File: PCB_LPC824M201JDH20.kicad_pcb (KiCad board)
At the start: 2 copper layers, 15.2 x 25.4 mm, 9 parts, among them J1 Conn_01x10, J2 Conn_01x10, U1 LPC824M201JDH20

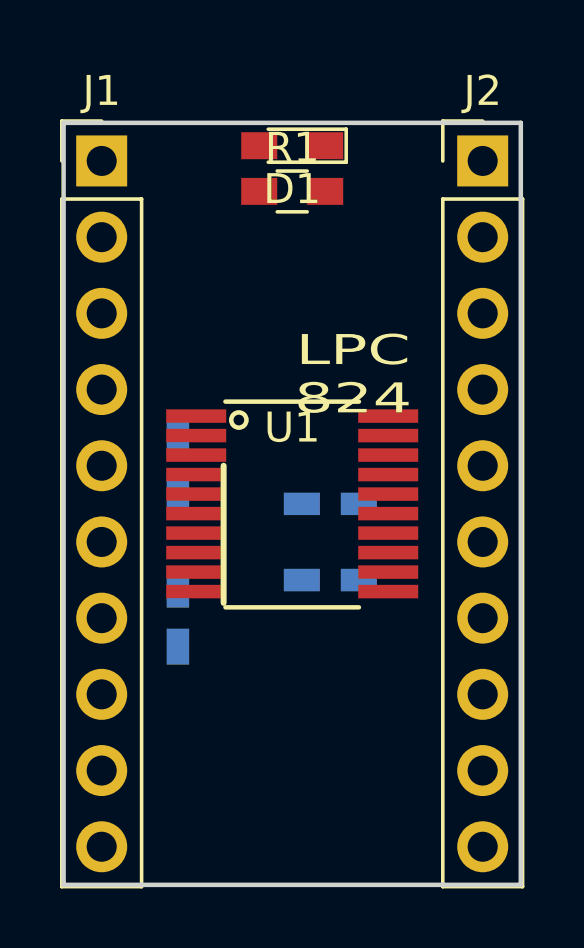
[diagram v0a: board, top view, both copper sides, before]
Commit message: no comment
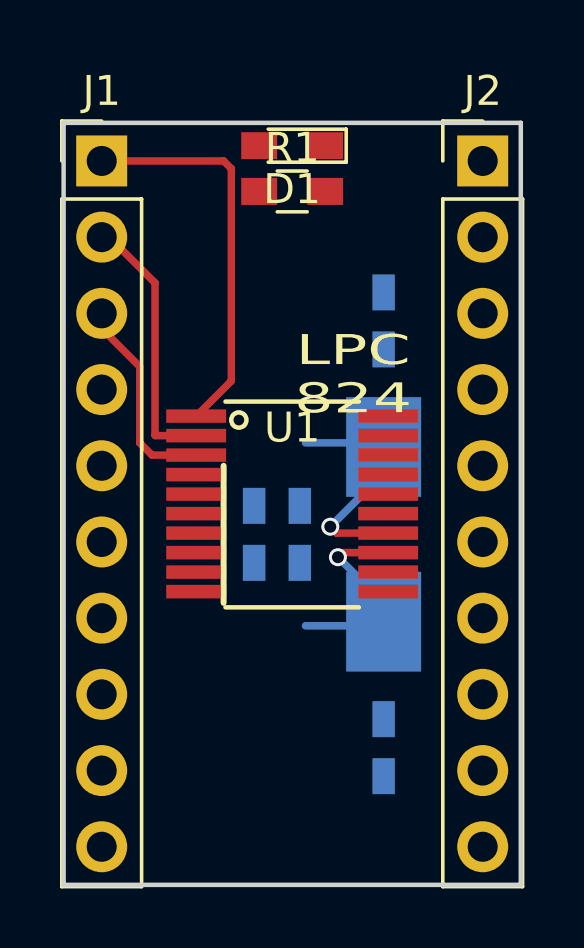
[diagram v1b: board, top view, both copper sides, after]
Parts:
- added 12MHz1: Crystal, Crystals:Crystal_SMD_0603-2pin_6.0x3.5mm_HandSoldering, B.Cu at (151.6, 111.5)
- moved C3 6.35 mm to (151.6, 104.4), turned to 270 degrees
- moved C4 5.86 mm to (151.6, 118.6), turned to 90 degrees
- moved C2 4.93 mm to (148.8, 111.5)
- moved C1 3.42 mm to (147.3, 111.5)
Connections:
- net Net-(J2-Pad3) renamed VREFP
- net Net-(J2-Pad4) renamed VREFN
- net Net-(J2-Pad5) renamed VSS
- net Net-(J2-Pad6) renamed VDD
- net RESET renamed PIO0_5
- J2 pad 1: Net-(J2-Pad1) -> PIO0_14
- J2 pad 10: Net-(J2-Pad10) -> PIO0_15
- J2 pad 2: Net-(J2-Pad2) -> PIO0_0
- J2 pad 7: Net-(J2-Pad7) -> XTALIN
- J2 pad 8: Net-(J2-Pad8) -> XTALOUT
- J2 pad 9: Net-(J2-Pad9) -> PIO0_1
- U1 pad 10: Net-(U1-Pad10) -> PIO0_10
- U1 pad 11: RFM_RST -> PIO0_15
- U1 pad 12: SCK -> PIO0_1
- U1 pad 19: RXD -> PIO0_0
- U1 pad 20: RFM_CS -> PIO0_14
- U1 pad 6: TXD -> PIO0_4
- U1 pad 7: SWCLK -> PIO0_3
- U1 pad 8: SWDIO -> PIO0_2
- U1 pad 9: FLASH_CS -> PIO0_11
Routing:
- net PIO0_23: track 0.00 -> 13.2 mm
- net PIO0_17: track 0.00 -> 8.87 mm
- net XTALIN: track 0.00 -> 8.08 mm, vias 0 -> 1
- net XTALOUT: track 0.00 -> 7.18 mm, vias 0 -> 1
- net PIO0_13: track 0.00 -> 6.89 mm

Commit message: no comment
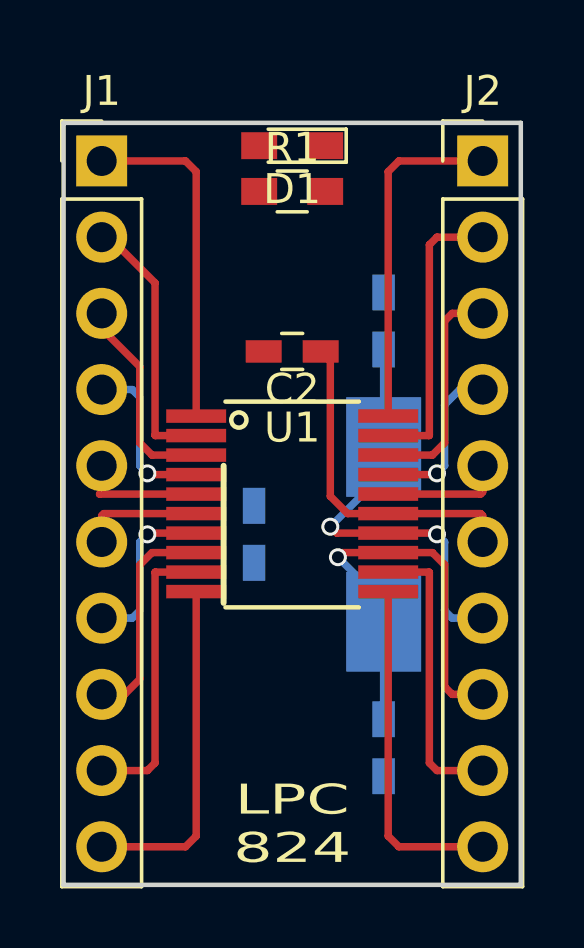
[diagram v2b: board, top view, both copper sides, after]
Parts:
- C2: moved to F.Cu
- moved C2 6.10 mm to (148.6, 105.4), turned to 180 degrees
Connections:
- J1 pad 5: PIO0_6 -> PIO0_5
- J2 pad 5: VSS -> GND
- J2 pad 6: VDD -> 3.3V
- U1 pad 17: GND -> VREFN
- U1 pad 18: 3.3V -> VREFP
- U1 pad 4: ISPE -> PIO0_12
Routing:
- net PIO0_14: track 0.00 -> 11.4 mm
- net PIO0_15: track 0.00 -> 11.4 mm
- net PIO0_10: track 0.00 -> 11.4 mm
- net 3.3V: track 0.00 -> 11.2 mm
- net PIO0_0: track 0.00 -> 9.61 mm
- net PIO0_1: track 0.00 -> 9.61 mm
- net PIO0_11: track 0.00 -> 9.61 mm
- net XTALOUT: track 7.18 -> 15.5 mm
- net VREFP: track 0.00 -> 7.49 mm
- net PIO0_2: track 0.00 -> 7.34 mm
- net XTALIN: track 8.08 -> 14.5 mm, vias 1 -> 2
- net PIO0_3: track 0.00 -> 5.66 mm, vias 0 -> 1
- net PIO0_12: track 0.00 -> 5.66 mm, vias 0 -> 1
- net VREFN: track 0.00 -> 5.51 mm, vias 0 -> 1
- net PIO0_5: track 0.00 -> 4.20 mm
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- added copper zone on B.Cu, net GND

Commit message: no comment
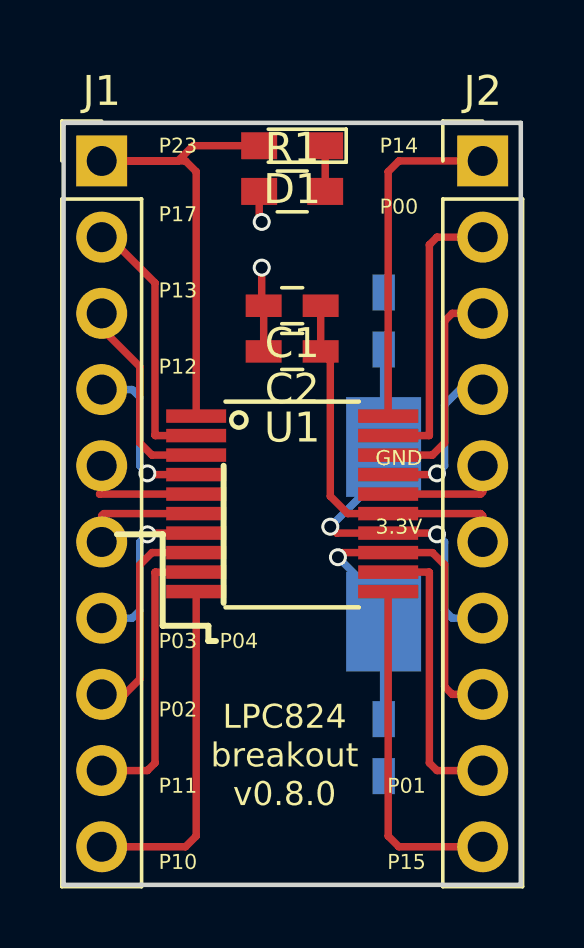
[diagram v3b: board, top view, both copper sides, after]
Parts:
- C1: moved to F.Cu
- moved C1 7.73 mm to (148.6, 103.9), turned to 180 degrees
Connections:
- J1 pad 1: PIO0_23 -> LED
- U1 pad 1: PIO0_23 -> LED
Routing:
- net LED: track 0.00 -> 16.9 mm
- net PIO0_23: track 11.4 -> 0.00 mm
- net GND: track 4.05 -> 7.93 mm, vias 0 -> 2
- net 3.3V: track 11.2 -> 12.7 mm
- net Net-(D1-Pad1): track 0.00 -> 1.52 mm
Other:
- board text added: "3.3V"
- board text added: "GND"
- board text added: "LPC824 breakout v0.8.0"
- board text added: "P00"
- board text added: "P01"
- board text added: "P02"
- board text added: "P03"
- board text added: "P04"
- board text added: "P10"
- board text added: "P11"
- board text added: "P12"
- board text added: "P13"
- board text added: "P14"
- board text added: "P15"
- board text added: "P17"
- board text added: "P23"
- board text removed: "LPC 824"
